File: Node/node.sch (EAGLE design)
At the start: 52 parts, among them SW1 SWITCH-MOMENTARY-2PTH, SW2 SWITCH-MOMENTARY-2PTH, SW3 SWITCH-MOMENTARY-2PTH, U1 FT232RLSSOP, U2 DW1000-I, U4 ATMEGA328, X2 332-02, Y1 8MHz, Y2 38.4MHz, 10pF

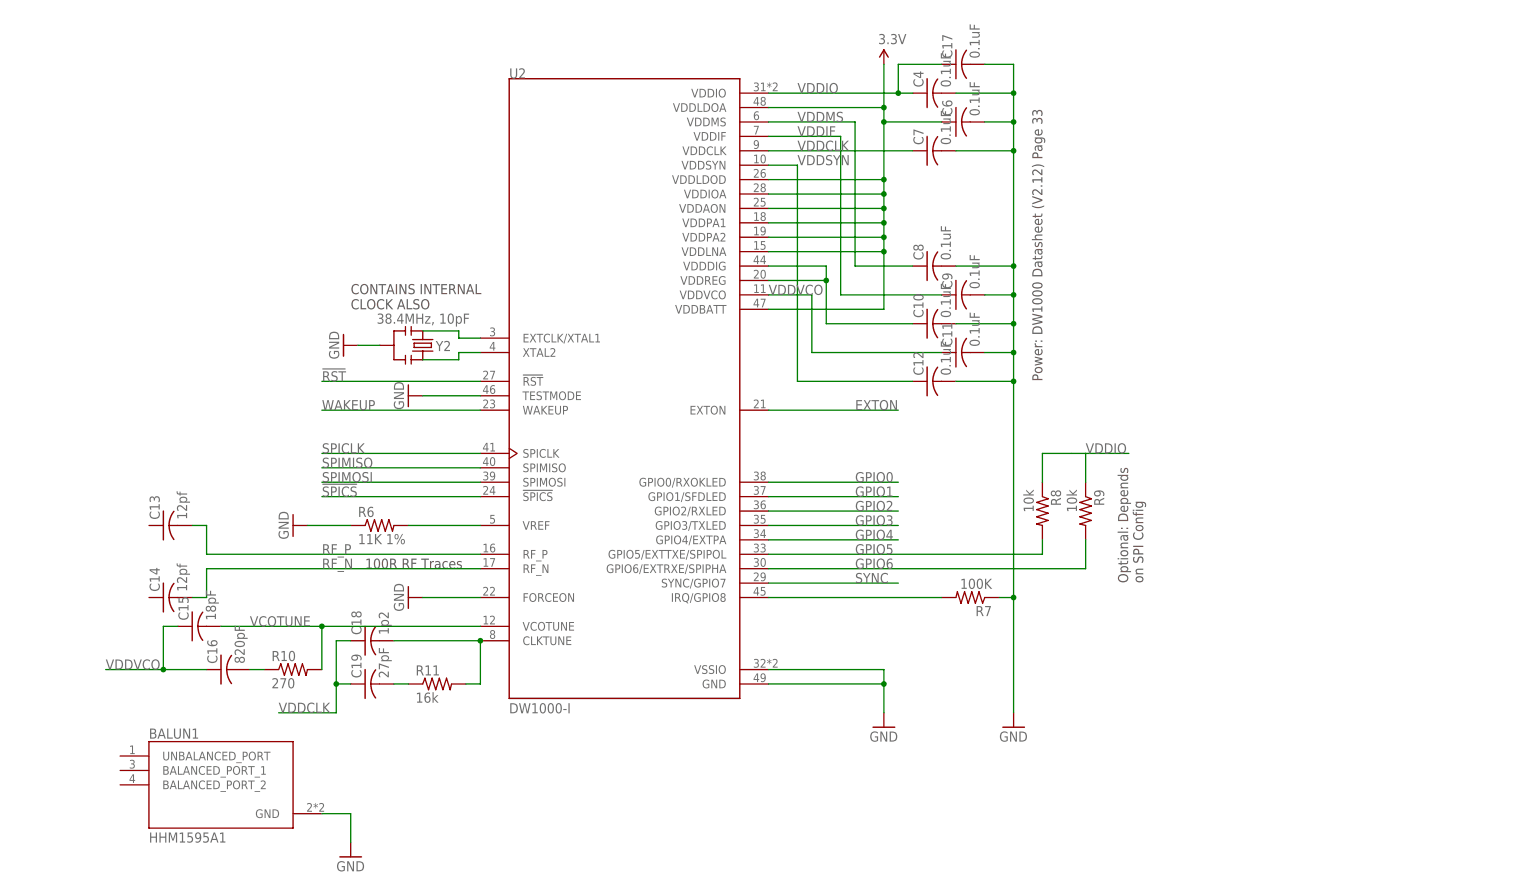
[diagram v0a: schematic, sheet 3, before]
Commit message: More work on schematic, documentation, frame, shielding, etc.
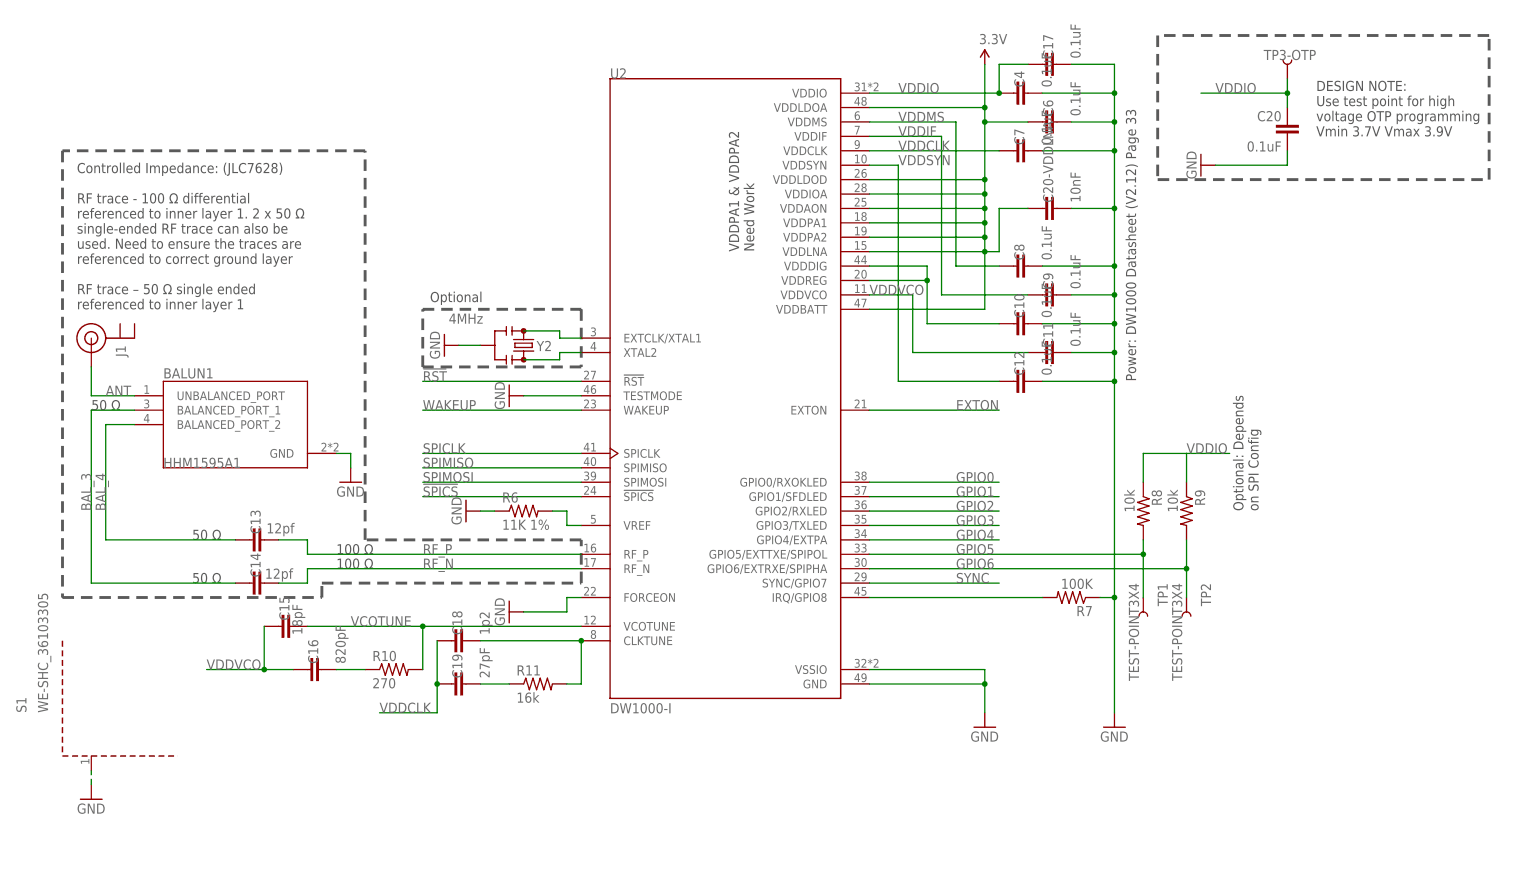
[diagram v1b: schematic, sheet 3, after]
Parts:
- added C20: 0.1uF, SparkFun-Passives:CAP0603-CAP
- added C20-VDDLNA: 10nF, SparkFun-Passives:CAP0603-CAP
- added J1: U.FL, SparkFun-Connectors:U.FL
- added S1: WE-SHC_36103305, Wurth_Elektronik_Passive_rev15e:WE-SHC_36103305
- added TP1, TP2, TP3-OTP: TEST-POINT3X4, SparkFun-Passives:TEST-POINT3X4
- C10, C11, C12, C13, C14, C15, C16, C17, C18, C19, C4, C6, C7, C8, C9: device adafruit:C-USC0603K -> SparkFun-Passives:CAP0603-CAP
- Y1: value 8MHz -> 4MHz; device SparkFun-FreqCtrl:RESONATORSMD -> SparkFun-FreqCtrl:RESONATOR4MHZ
- Y2: value 38.4MHz, 10pF -> 4MHz; device SparkFun-FreqCtrl:RESONATORSMD -> SparkFun-FreqCtrl:RESONATOR4MHZ
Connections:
- new net ANT: BALUN1.UNBALANCED_PORT, J1.SIGNAL
- new net BAL_3: BALUN1.BALANCED_PORT_1, C14.1
- new net BAL_4: BALUN1.BALANCED_PORT_2, C13.1
- net 3.3V: now also C20-VDDLNA.1
- net GND: now also C20-VDDLNA.2, C20.1, S1.GND
- net GPIO5: now also TP1.1
- net GPIO6: now also TP2.1
- net VDDIO: now also C20.2, TP3-OTP.1
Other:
- note added: "100 Ω"
- note added: "50 Ω"
- note added: "Controlled Impedance: (JLC7628) RF trace - 100 Ω differential referenced to inner layer 1. 2 x 50 Ω single-ended RF trace can also be used. Need to ensure the traces are referenced to correct ground layer RF trace – 50 Ω single ended referenced to inner layer 1"
- note added: "DESIGN NOTE: Use test point for high voltage OTP programming Vmin 3.7V Vmax 3.9V"
- note added: "Optional"
- note added: "VDDPA1 & VDDPA2 Need Work"
- note removed: "100R RF Traces"
- note removed: "CONTAINS INTERNAL CLOCK ALSO"
- moved on the sheet: BALUN1, C10, C11, C12, C13, C14, C15, C16, C17, C18, C19, C4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
